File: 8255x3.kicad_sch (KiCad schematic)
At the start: 7 parts

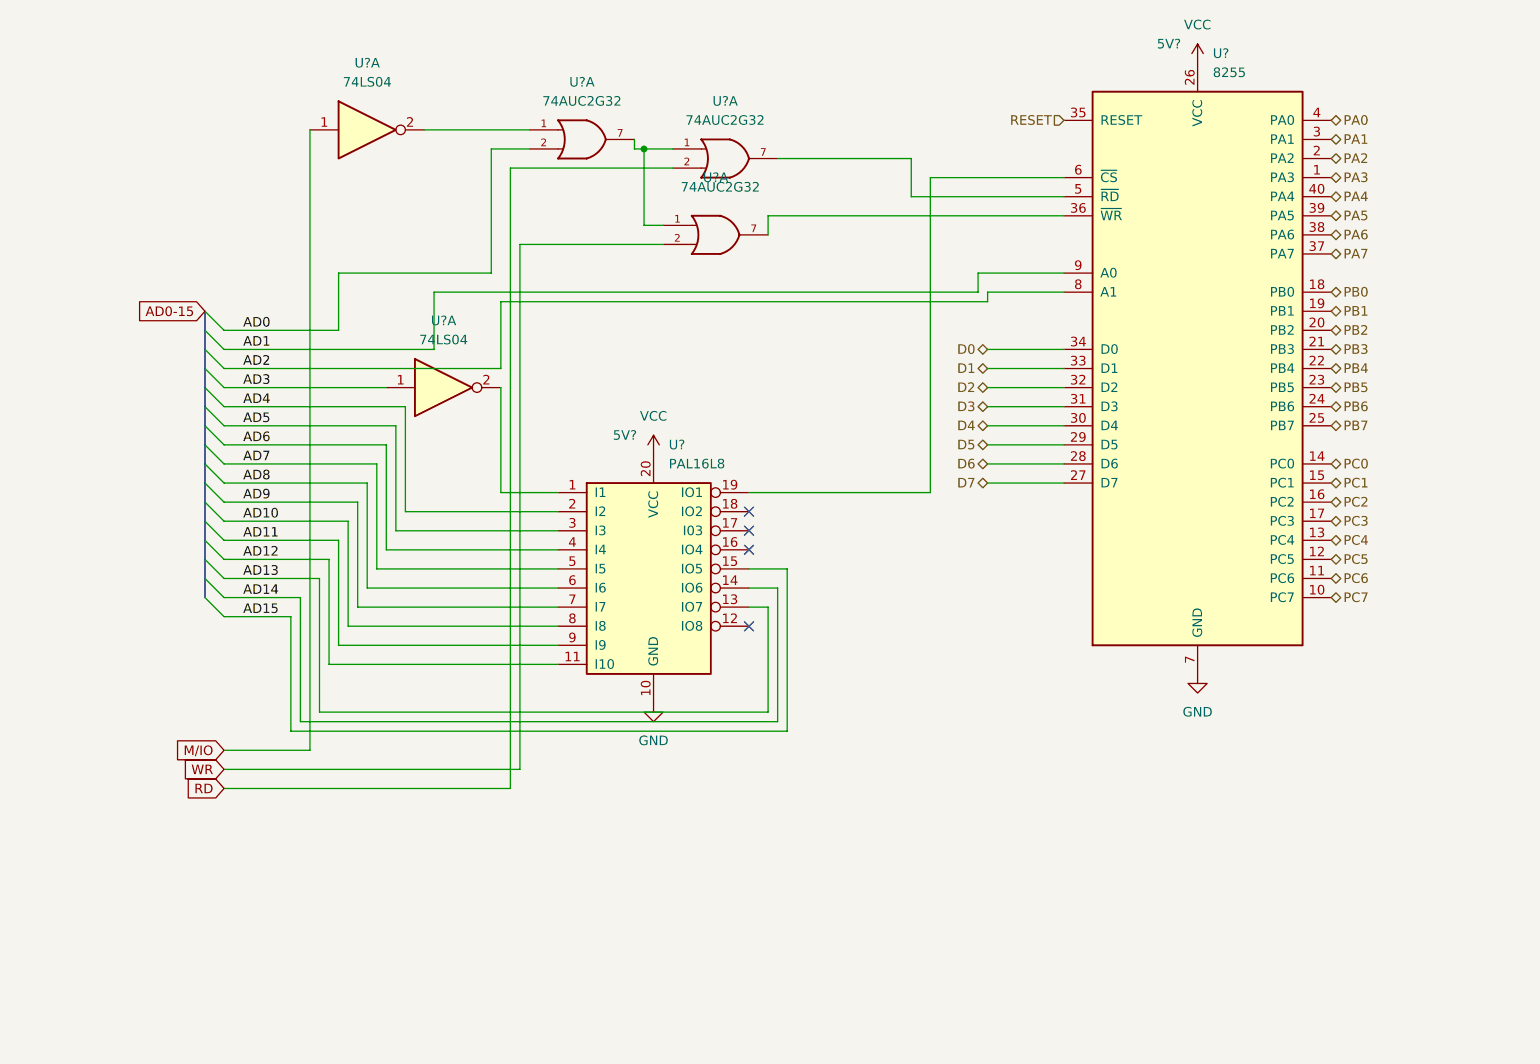
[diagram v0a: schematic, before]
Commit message: Add files via upload
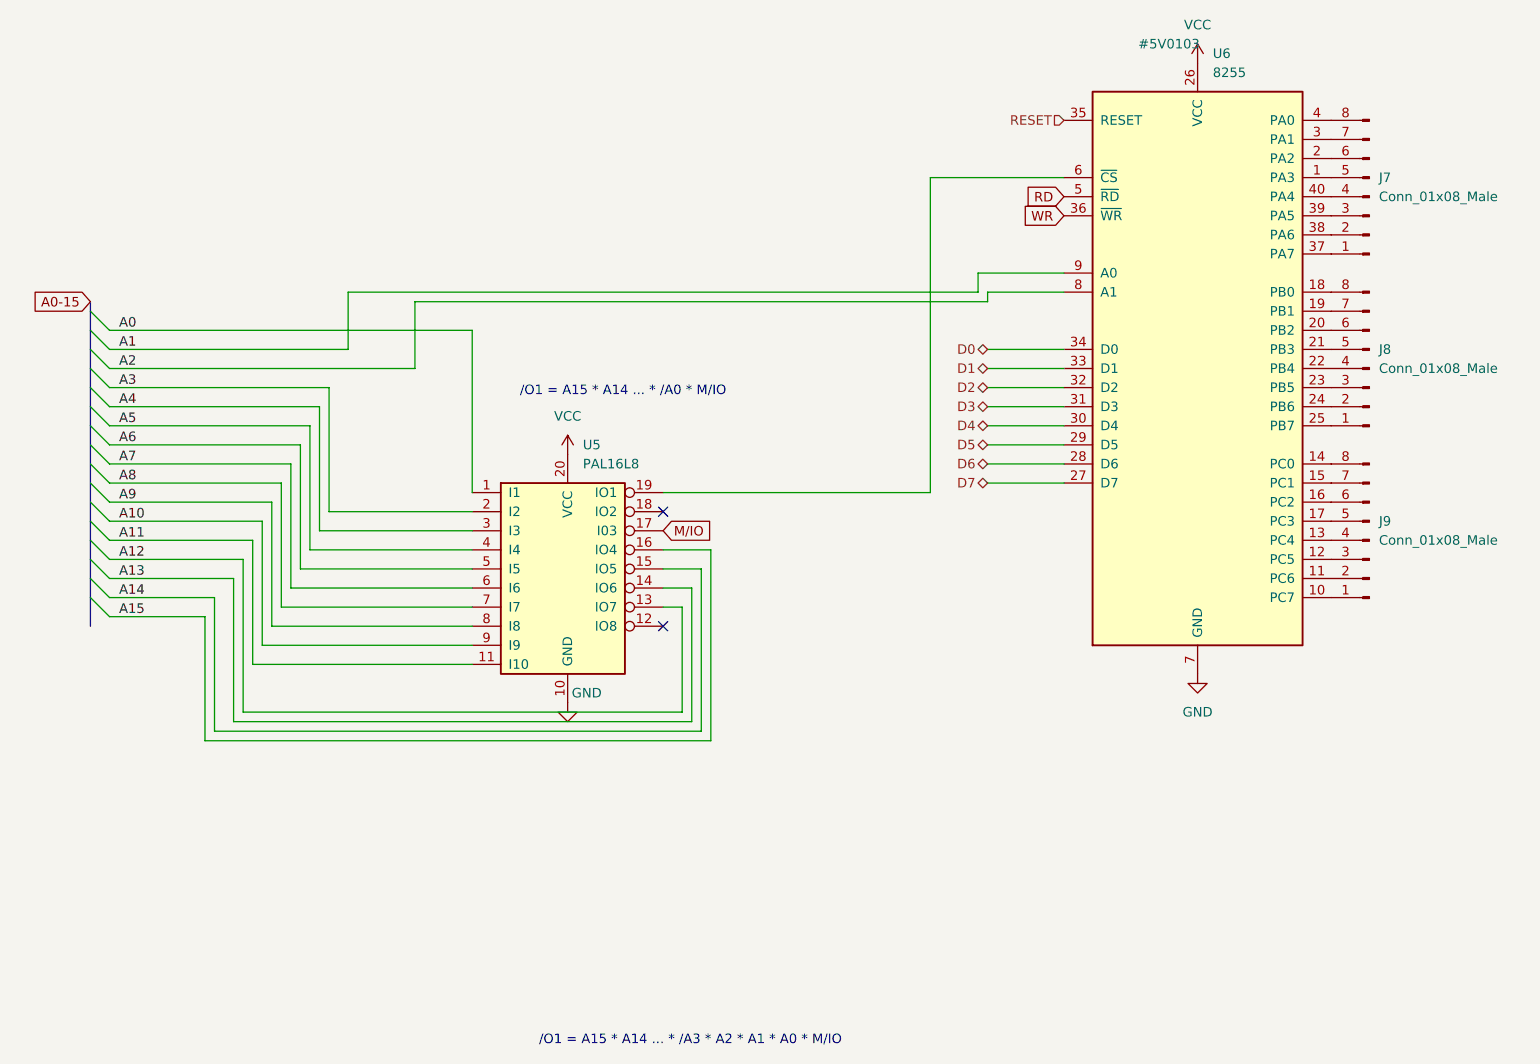
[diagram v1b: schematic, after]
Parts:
- removed U? (x3): 74AUC2G32, symbol 74xGxx:74AUC2G32
- removed U? (x2): 74LS04, symbol 74xx:74LS04
- removed U?: PAL16L8, symbol Logic_Programmable:PAL16L8
- added J7, J8, J9: Conn_01x08_Male, symbol Connector:Conn_01x08_Male
- added U5: PAL16L8, symbol Logic_Programmable:PAL16L8
- gave numbers to parts that had none: 1
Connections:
- net GND: now also U5.10 (GND)
- net M/IO: now also U5.17 (I03)
- net RD: now also U6.5 (~{RD})
- net VCC: now also U5.20 (VCC)
- net WR: now also U6.36 (~{WR})
- net at U6.6 (~{CS}): now also U5.19 (IO1)
- net AD1 renamed A1
- net AD2 renamed A2
- net PA0: no longer names the net of U6.4 (PA0)
- net PA0: now also J7.8 (Pin_8)
- net PA1: no longer names the net of U6.3 (PA1)
- net PA1: now also J7.7 (Pin_7)
- net PA2: no longer names the net of U6.2 (PA2)
- net PA2: now also J7.6 (Pin_6)
- net PA3: no longer names the net of U6.1 (PA3)
- net PA3: now also J7.5 (Pin_5)
- net PA4: no longer names the net of U6.40 (PA4)
- net PA4: now also J7.4 (Pin_4)
- net PA5: no longer names the net of U6.39 (PA5)
- net PA5: now also J7.3 (Pin_3)
- net PA6: no longer names the net of U6.38 (PA6)
- net PA6: now also J7.2 (Pin_2)
- net PA7: no longer names the net of U6.37 (PA7)
- net PA7: now also J7.1 (Pin_1)
- net PB0: no longer names the net of U6.18 (PB0)
- net PB0: now also J8.8 (Pin_8)
- net PB1: no longer names the net of U6.19 (PB1)
- net PB1: now also J8.7 (Pin_7)
- net PB2: no longer names the net of U6.20 (PB2)
- net PB2: now also J8.6 (Pin_6)
- net PB3: no longer names the net of U6.21 (PB3)
- net PB3: now also J8.5 (Pin_5)
- net PB4: no longer names the net of U6.22 (PB4)
- net PB4: now also J8.4 (Pin_4)
- net PB5: no longer names the net of U6.23 (PB5)
- net PB5: now also J8.3 (Pin_3)
- net PB6: no longer names the net of U6.24 (PB6)
- net PB6: now also J8.2 (Pin_2)
- net PB7: no longer names the net of U6.25 (PB7)
- net PB7: now also J8.1 (Pin_1)
- net PC0: no longer names the net of U6.14 (PC0)
- net PC0: now also J9.8 (Pin_8)
- net PC1: no longer names the net of U6.15 (PC1)
- net PC1: now also J9.7 (Pin_7)
- net PC2: no longer names the net of U6.16 (PC2)
- net PC2: now also J9.6 (Pin_6)
- net PC3: no longer names the net of U6.17 (PC3)
- net PC3: now also J9.5 (Pin_5)
- net PC4: no longer names the net of U6.13 (PC4)
- net PC4: now also J9.4 (Pin_4)
- net PC5: no longer names the net of U6.12 (PC5)
- net PC5: now also J9.3 (Pin_3)
- net PC6: no longer names the net of U6.11 (PC6)
- net PC6: now also J9.2 (Pin_2)
- net PC7: no longer names the net of U6.10 (PC7)
- net PC7: now also J9.1 (Pin_1)
- new net A0: U5.1 (I1)
- new net A10: U5.9 (I9)
- new net A11: U5.11 (I10)
- new net A12: U5.13 (IO7)
- new net A13: U5.14 (IO6)
- new net A14: U5.15 (IO5)
- new net A15: U5.16 (IO4)
- new net A3: U5.2 (I2)
- new net A4: U5.3 (I3)
- new net A5: U5.4 (I4)
- new net A6: U5.5 (I5)
- new net A7: U5.6 (I6)
- new net A8: U5.7 (I7)
- new net A9: U5.8 (I8)
- no-connect marks 4 -> 2
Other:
- note added: "/O1 = A15 * A14 ... * /A0 * M/IO"
- note added: "/O1 = A15 * A14 ... * /A3 * A2 * A1 * A0 * M/IO"
